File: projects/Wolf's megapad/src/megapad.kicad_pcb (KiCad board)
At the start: 2 copper layers, 127.5 x 54.5 mm, 85 parts, among them Q1 AO3415AL, Q2 AO3415AL, Q3 AO3415AL, Q4 AO3415AL, Q5 AO3415AL, SW1 MX1A-11NW, SW2 MX1A-11NW, SW3 MX1A-11NW, SW4 MX1A-11NW, SW5 MX1A-11NW, SW6 MX1A-11NW, U1 SL2.1A_C6798314, U2 TS3USB221RSER, U3 W25Q80DVSNIG, U4 X322512MSB4SI, U5 RP2040, U6 NCP1117ST33T3G

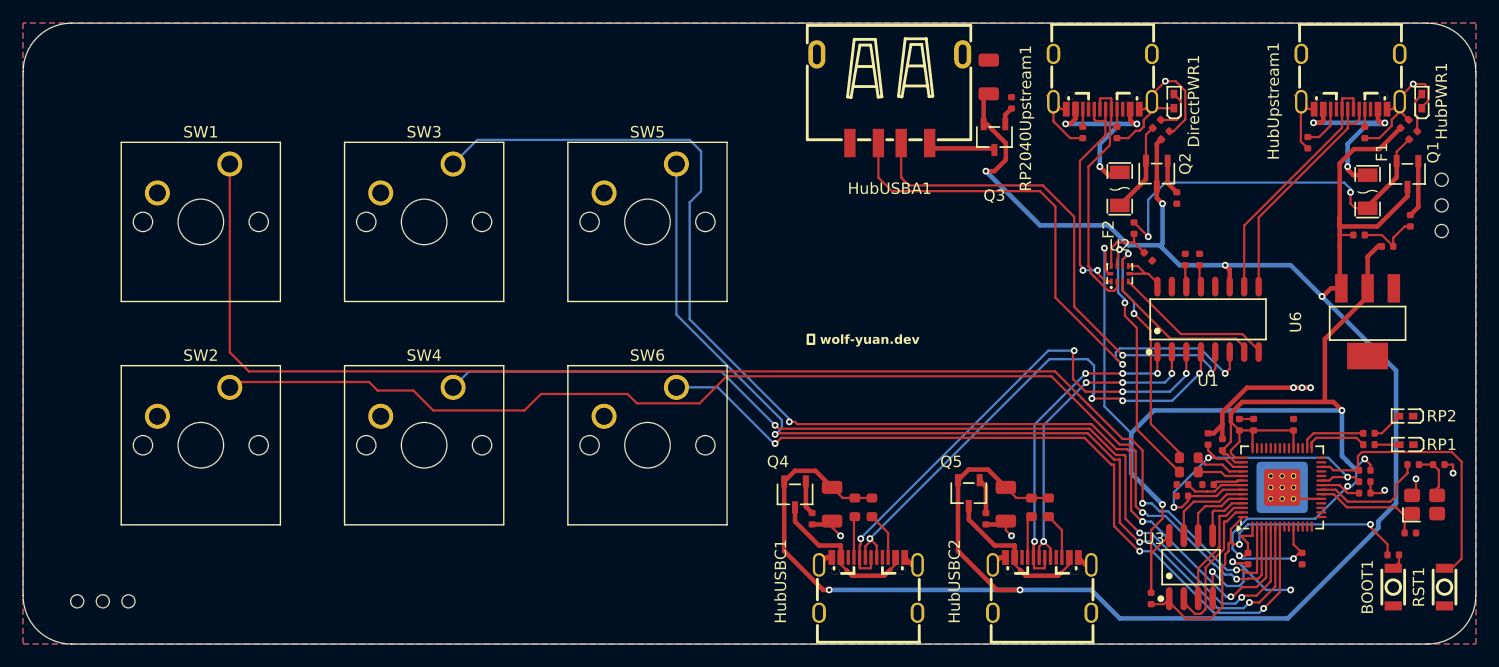
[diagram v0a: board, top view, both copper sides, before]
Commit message: feat: update megapad design and schematic
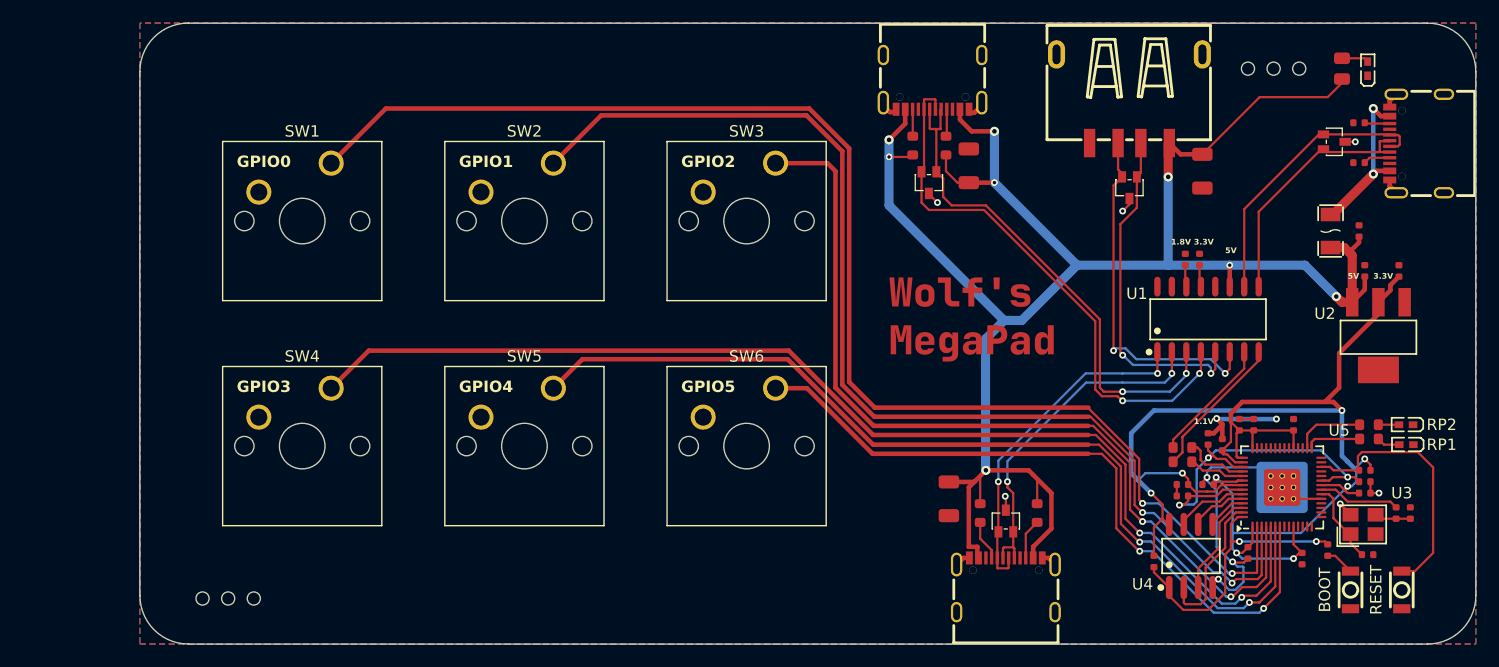
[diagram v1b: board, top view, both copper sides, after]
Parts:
- removed the C11 at (301.8, 100.3)
- removed DirectPWR1: FC-F1005WD-455K5, easyeda2kicad:LED0402-R-RD
- removed F2: SMD1206P150TF, easyeda2kicad:F1206
- removed Q1, Q2, Q3, Q4, Q5: AO3415AL, easyeda2kicad:SOT-23-3_L2.9-W1.6-P1.90-LS2.9-BL
- removed the R11 at (297.5, 100.1)
- removed the R12 at (299.0, 108.5)
- removed the R13 at (301.0, 99.3)
- removed the R14 at (300.2, 111.0)
- removed R21, R22, R23, R24, R25: 100kΩ, PCM_JLCPCB:R_0402
- removed the R8 at (294.5, 100.1)
- removed RP2040Upstream1: USB3.1C16PFSMT, easyeda2kicad:USB-C-SMD_TYPE-C-USB-17
- removed the U2 at (297.8, 112.5)
- added D1: TPD2E2U06DCKR, easyeda2kicad:SC-70-3_L2.0-W1.3-P0.65-LS2.1-BL, F.Cu at (316.6, 100.9)
- added D2: TPD2E2U06DCKR, easyeda2kicad:SC-70-3_L2.0-W1.3-P0.65-LS2.1-BL, F.Cu at (298.6, 105.0)
- added D3: TPD2E2U06DCKR, easyeda2kicad:SC-70-3_L2.0-W1.3-P0.65-LS2.1-BL, F.Cu at (287.8, 134.2)
- added D4: TPD2E2U06DCKR, easyeda2kicad:SC-70-3_L2.0-W1.3-P0.65-LS2.1-BL, F.Cu at (281.0, 104.5)
- HubUSBA1: value AF 10.0 HC6.3 -> USB-AF-90-10X14.4-H6.57
- HubUSBC1, HubUSBC2, HubUpstream1: value USB3.1C16PFSMT -> MC-311D; footprint easyeda2kicad:USB-C-SMD_TYPE-C-USB-17 -> easyeda2kicad:USB-C-SMD_MC-311D
- R14: renamed from R19; value 200Ω -> 47Ω; footprint PCM_JLCPCB:R_0402 -> PCM_JLCPCB:R_0603
- R15: renamed from R20; value 200Ω -> 47Ω; footprint PCM_JLCPCB:R_0402 -> PCM_JLCPCB:R_0603
- R7: value 200Ω -> 150Ω; footprint PCM_JLCPCB:R_0402 -> PCM_JLCPCB:R_0805
- U3: renamed from U4; value X322512MSB4SI -> ABM8-272-T3_C20625731; footprint PCM_JLCPCB:CRYSTAL-SMD_4P-L3.2-W2.5-BL -> easyeda2kicad:CRYSTAL-SMD_4P-L3.2-W2.5-BL
- moved HubUSBC1 44.5 mm to (281.3, 95.7), turned to 180 degrees
- moved SW2 34.5 mm to (248.0, 102.8)
- moved R2 32.4 mm to (282.5, 101.2), turned to 90 degrees
- moved R5 32.2 mm to (279.6, 101.2), turned to 90 degrees
- moved C4 32.0 mm to (284.5, 103.0), turned to -90 degrees
- moved SW3 28.3 mm to (267.5, 102.8)
- moved SW5 22.4 mm to (248.0, 122.5)
- moved HubUSBA1 21.0 mm to (298.6, 97.1)
- moved C1 20.5 mm to (305.0, 103.5), turned to 90 degrees
- moved ? 19.6 mm to (309.0, 94.5), turned to 180 degrees
- moved REF** 19.0 mm to (311.2, 94.5), turned to 180 degrees
- moved ? 19.0 mm to (313.5, 94.5), turned to 180 degrees
- moved ? 11.0 mm to (217.2, 141.0)
- moved ? 11.0 mm to (221.8, 141.0)
- moved REF** 11.0 mm to (219.5, 141.0)
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- renumbered C14 to C11, C15 to C12, C16 to C13, C17 to C14, C18 to C15, C19 to C16, C20 to C17, C21 to C18, C22 to C19, C6 to C2, C23 to C20, C24 to C21, C25 to C22, C7 to C3, C8 to C6, C12 to C7, C9 to C8, C13 to C9, R15 to R10, R16 to R11, R17 to R12, R18 to R13, R6 to R4, R4 to R5, R5 to R6, R9 to R8, R10 to R9, U6 to U2, U3 to U4
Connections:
- F1 pad 2: /5VDET -> +5V
- HubUSBA1 pad 1: Net-(HubUSBA1-VCC) -> +5V
- HubUSBA1 pad 5: (no net) -> GND
- HubUSBA1 pad 6: (no net) -> GND
- R1 pad 2: Net-(HubUpstream1-CC2) -> Net-(HubUpstream1-CC1)
- R11 pad 1: Net-(U2-D+) -> /HubRP2040+
- R12 pad 1: Net-(U2-D-) -> /HubRP2040-
- R2 pad 2: Net-(HubUSBC1-CC2) -> Net-(HubUSBC1-CC1)
- R3 pad 2: Net-(HubUSBC2-CC2) -> Net-(HubUSBC2-CC1)
- R4 pad 2: Net-(HubUpstream1-CC1) -> Net-(HubUpstream1-CC2)
- R5 pad 2: Net-(HubUSBC1-CC1) -> Net-(HubUSBC1-CC2)
- R6 pad 2: Net-(HubUSBC2-CC1) -> Net-(HubUSBC2-CC2)
- R7 pad 1: /5VDET -> +5V
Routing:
- net GND: track 106.6 -> 53.6 mm, vias 13 -> 11
- net /5VDET: track 34.4 -> 0.00 mm, vias 2 -> 0
- net +5V: track 204.1 -> 170.5 mm, vias 6 -> 8
- net Net-(U5-GPIO2): track 107.3 -> 77.6 mm, vias 3 -> 2
- net Net-(U2-D+): track 23.3 -> 0.00 mm, vias 2 -> 0
- net /DirectD-: track 21.8 -> 0.00 mm
- net Net-(U2-D-): track 21.5 -> 0.00 mm, vias 2 -> 0
- net +3V3: track 154.6 -> 133.9 mm, vias 7 -> 8
- net /DirectD+: track 20.2 -> 0.00 mm, vias 2 -> 0
- net /HubUSBA1+: track 50.4 -> 31.9 mm
- net /VBUSDirect: track 17.1 -> 0.00 mm, vias 3 -> 0
- net Net-(Q4-D): track 14.5 -> 0.00 mm
- net Net-(Q5-D): track 14.4 -> 0.00 mm
- net /HubUSBA1-: track 44.5 -> 30.2 mm
- net Net-(U5-GPIO3): track 89.6 -> 101.4 mm, vias 3 -> 2
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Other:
- board size 127.5 x 54.5 mm -> 117.3 x 54.5 mm
- board text added: "1.1V"
- board text added: "1.8V"
- board text added: "3.3V"
- board text added: "5V"
- board text added: "GPIO0"
- board text added: "GPIO1"
- board text added: "GPIO2"
- board text added: "GPIO3"
- board text added: "GPIO4"
- board text added: "GPIO5"
- board text added: "USBA Out"
- board text added: "USBC Out1"
- board text added: "USBC Out2"
- board text added: "USBC Source"
- board text removed: "Wolf's MegaPad"
- board text removed: "󰖟 wolf-yuan.dev"
